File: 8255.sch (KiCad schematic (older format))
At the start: 16 parts, among them U7 PAL16L8

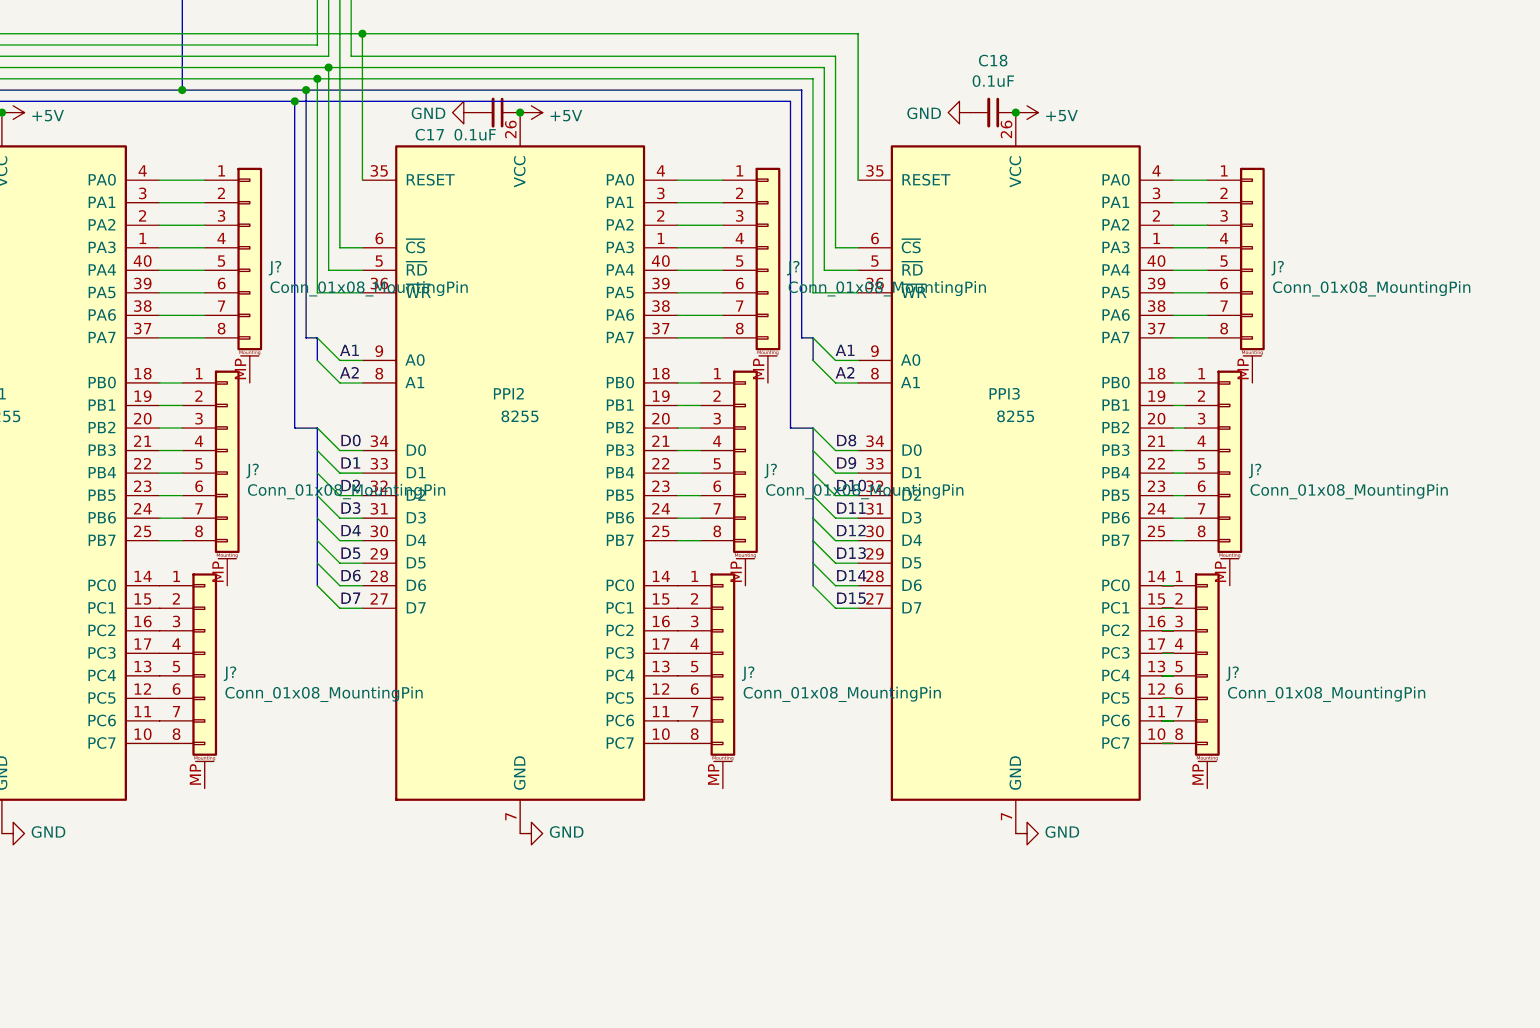
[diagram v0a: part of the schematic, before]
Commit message: Fixing Weirdness
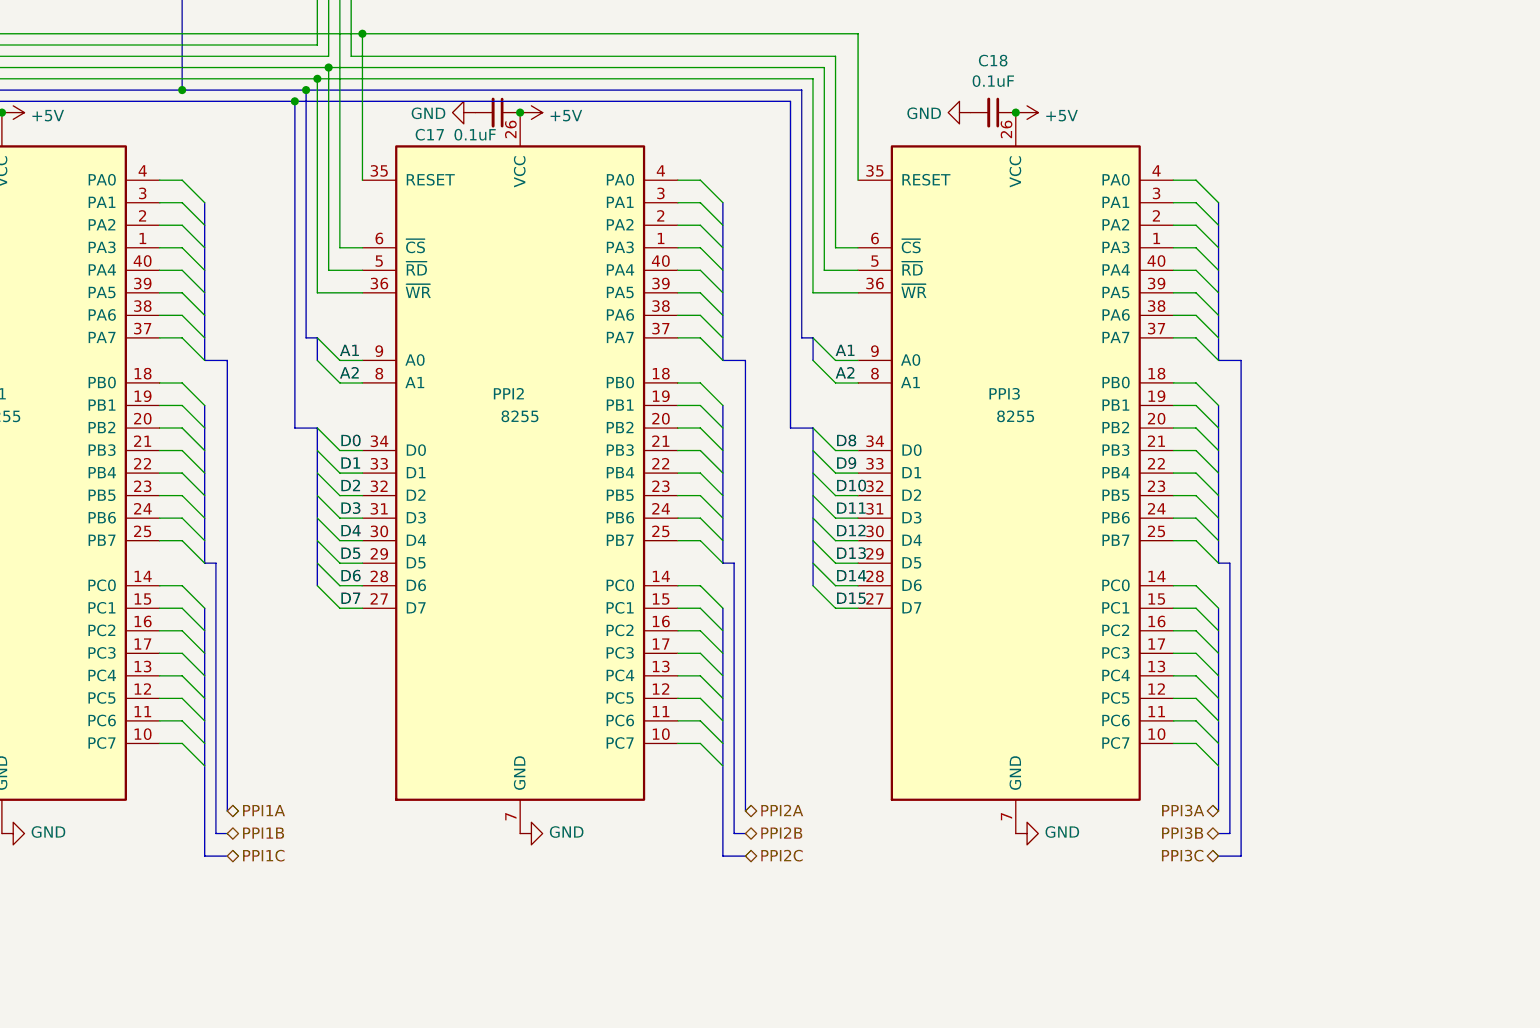
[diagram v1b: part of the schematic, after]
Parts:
- removed J? (x9): Conn_01x08_MountingPin, symbol Connector_Generic_MountingPin:Conn_01x08_MountingPin
